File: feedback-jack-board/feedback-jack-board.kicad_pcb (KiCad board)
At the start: 2 copper layers, 77.5 x 37 mm, 12 parts, among them J1 Out, J2 Ret, J3 In, J4 Snd, J5 FPC_Connector, J6 Barrel_Jack_Switch

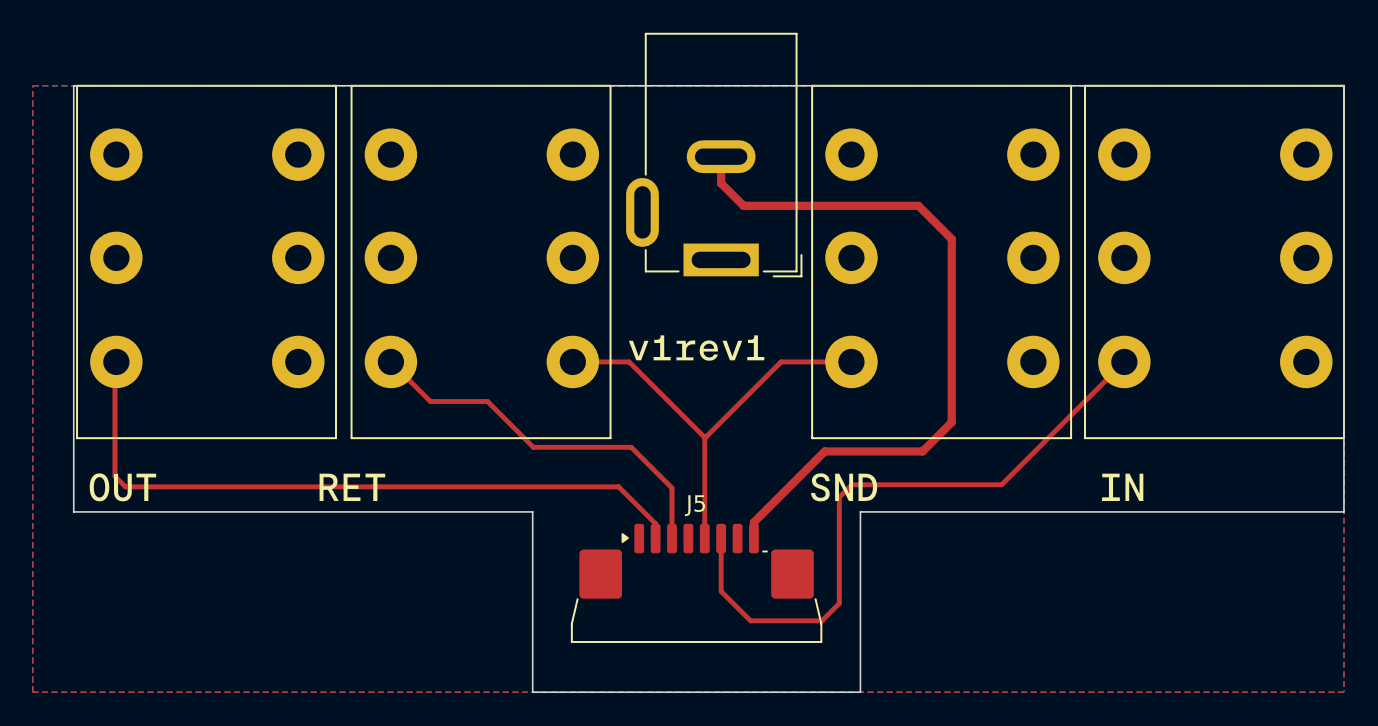
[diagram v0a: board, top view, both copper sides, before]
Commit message: Jacks board v2rev1
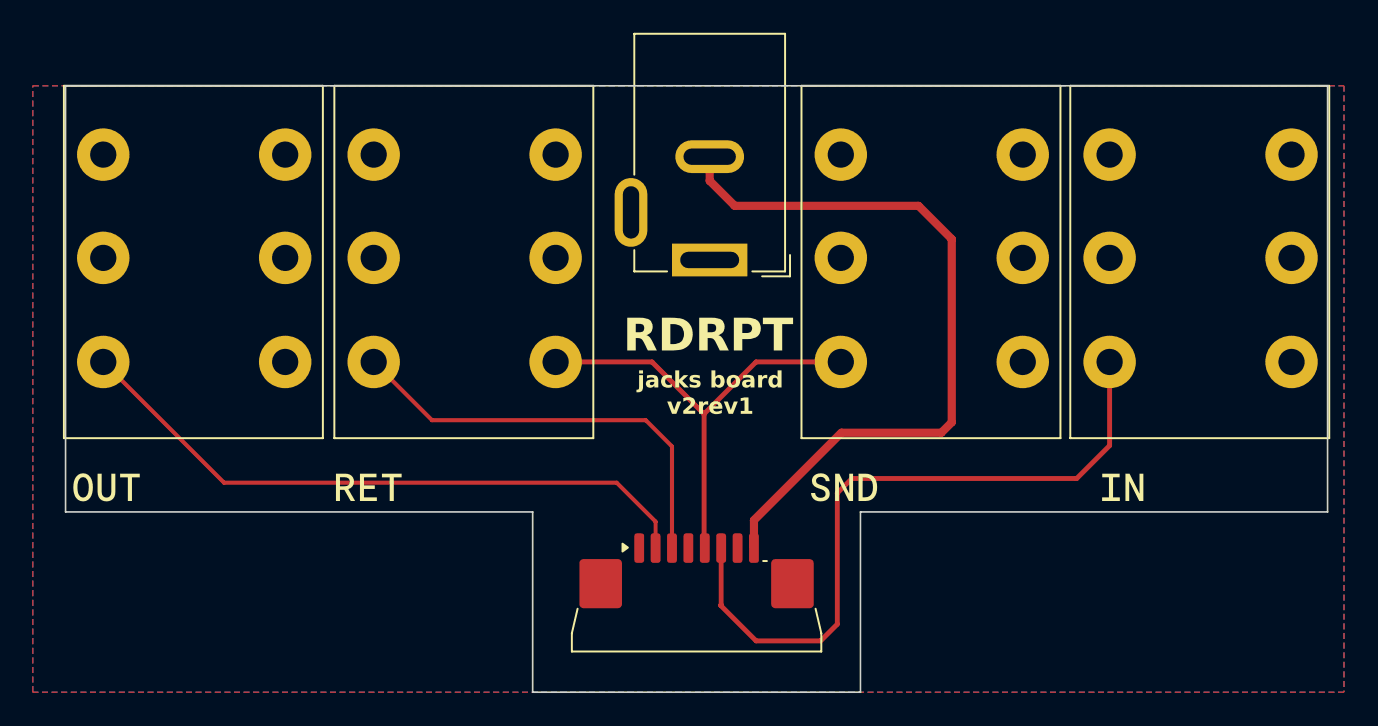
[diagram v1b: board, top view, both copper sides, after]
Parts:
- removed kibuzzard-67A4F0EE: G***, kibuzzard-67A4F0EE
- moved J2 1.05 mm to (87.2, 45.0)
- moved kibuzzard-67A4F113 1.00 mm to (64.0, 69.5)
- moved kibuzzard-67A4F12B 1.00 mm to (80.0, 69.5)
- moved J3 0.90 mm to (132.1, 45.0)
- moved J1 0.80 mm to (70.7, 45.0)
- moved J6 0.70 mm to (100.8, 55.6)
- moved J4 0.65 mm to (115.7, 45.0)
- moved J5 0.58 mm to (100.0, 76.6)
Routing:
- net /In: track 38.9 -> 42.9 mm
- net /Ret: track 23.4 -> 26.5 mm
- net /Out: track 42.1 -> 39.3 mm
- net /Snd: track 27.0 -> 28.9 mm
- net /Jack9V: track 43.9 -> 45.1 mm
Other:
- board size 77.5 x 37 mm -> 77 x 37 mm
- board text added: "RDRPT"
- board text added: "jacks board v2rev1"
